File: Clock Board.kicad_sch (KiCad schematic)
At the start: 20 parts, among them SW1 Micro Push SPST, SW2 SW_SPDT, U1 NE555P, U2 NE555P, U3 NE555P, U4 74HCT02, U5 74HCT02, U6 74LS08

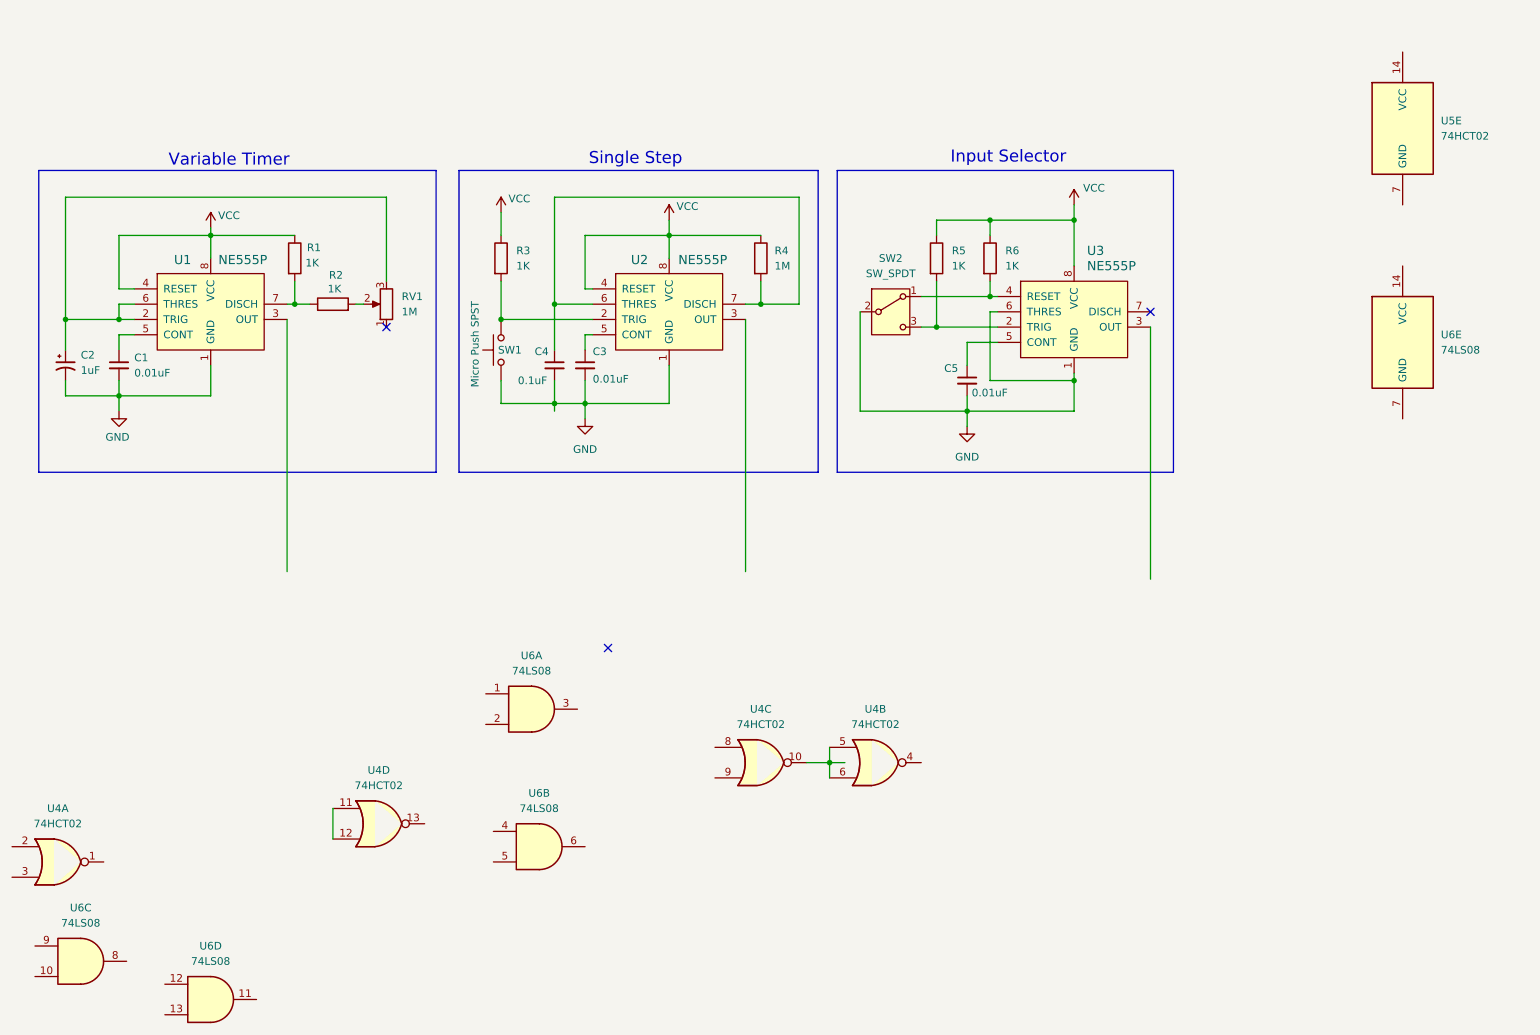
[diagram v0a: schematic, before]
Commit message: PCB Work
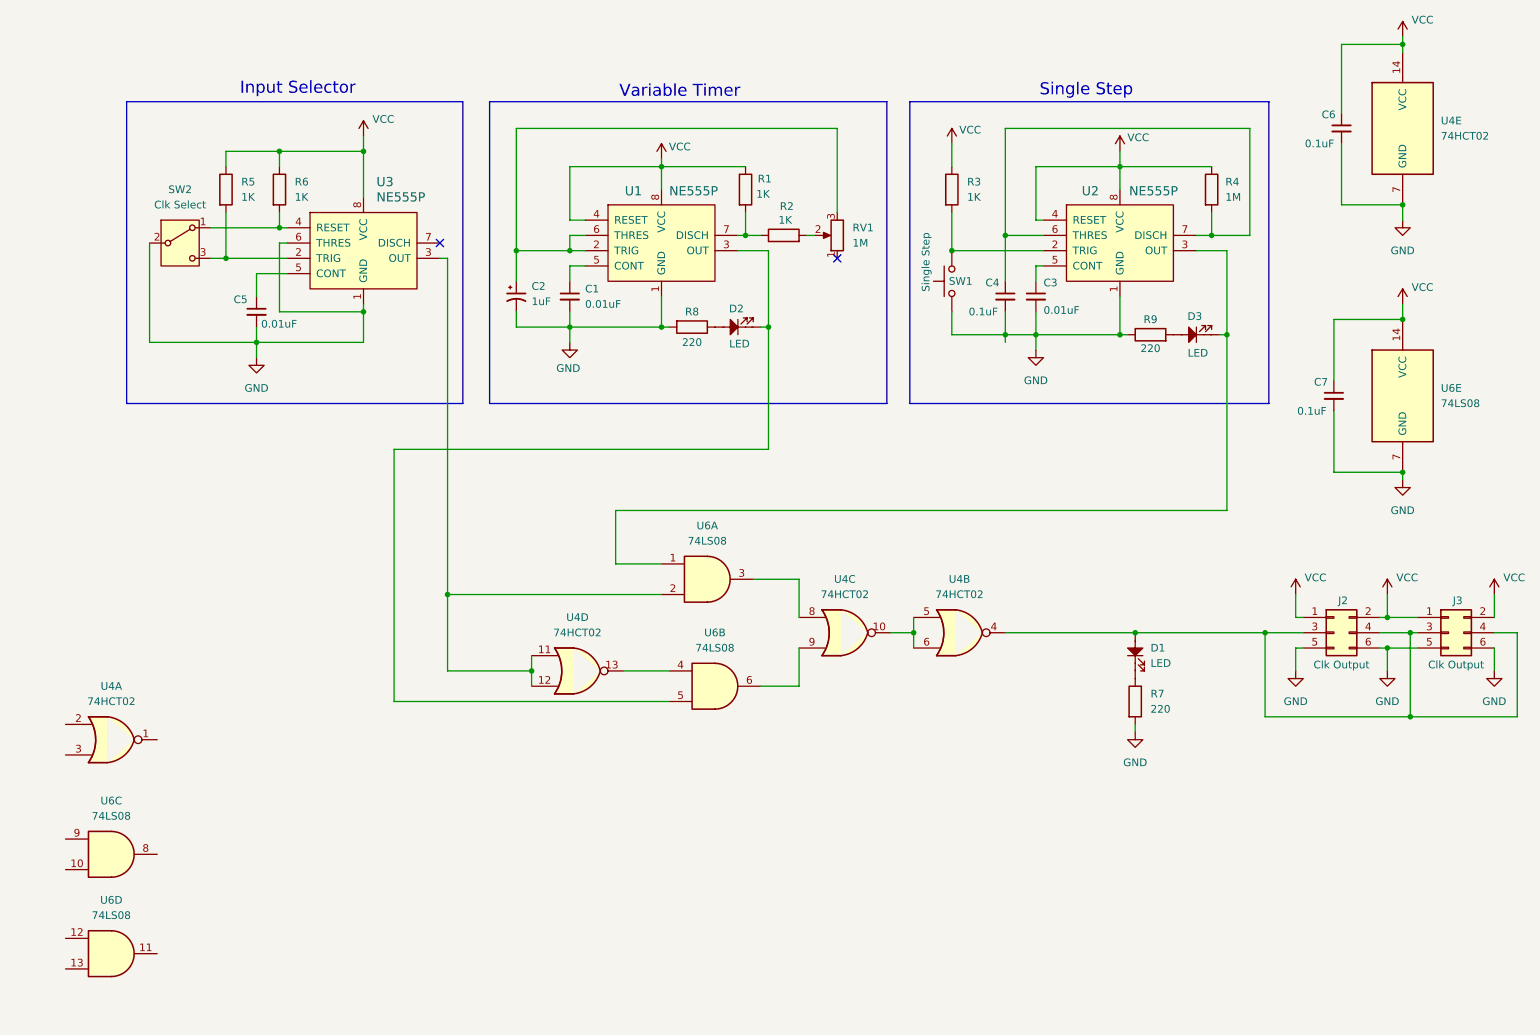
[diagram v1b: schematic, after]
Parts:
- added C6, C7: 0.1uF, Capacitor_THT:C_Disc_D5.0mm_W2.5mm_P5.00mm, symbol Device:C_Small
- added D1, D2, D3: LED, LED_THT:LED_D5.0mm, symbol PCM_SL_Devices:LED
- added J2: Clk Output, Connector_PinSocket_2.54mm:PinSocket_2x03_P2.54mm_Vertical, symbol Connector_Generic:Conn_02x03_Odd_Even
- added J3: Clk Output, Connector_PinHeader_2.54mm:PinHeader_2x03_P2.54mm_Vertical, symbol Connector_Generic:Conn_02x03_Odd_Even
- added R7, R8, R9: 220, Resistor_THT:R_Axial_DIN0207_L6.3mm_D2.5mm_P10.16mm_Horizontal, symbol Device:R
- C1, C3, C4, C5: footprint (none) -> Capacitor_THT:C_Disc_D5.0mm_W2.5mm_P5.00mm
- C2: footprint (none) -> PCM_Capacitor_THT_AKL:CP_Radial_D5.0mm_P2.00mm
- R1, R2, R3, R4, R5, R6: footprint (none) -> Resistor_THT:R_Axial_DIN0207_L6.3mm_D2.5mm_P10.16mm_Horizontal
- RV1: footprint (none) -> Potentiometer_THT:Potentiometer_TT_P0915N
- SW1: value Micro Push SPST -> Single Step; footprint (none) -> digikey-footprints:Terminal_Block_D1.3mm_P5mm
- SW2: value SW_SPDT -> Clk Select; footprint (none) -> Button_Switch_THT:SW_Slide_SPDT_Straight_CK_OS102011MS2Q
- U1, U2, U3: footprint digikey-footprints:DIP-8_W7.62mm -> Package_DIP:DIP-8_W7.62mm_Socket
- U4, U6: footprint (none) -> Package_DIP:DIP-14_W7.62mm_Socket
- U4: renamed from U5; footprint (none) -> Package_DIP:DIP-14_W7.62mm_Socket
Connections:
- net GND: now also U4.7 (GND), U6.7 (GND), C6.2, C7.2, J2.5 (Pin_5), J2.6 (Pin_6), J3.5 (Pin_5), J3.6 (Pin_6), R7.2, R8.2, R9.1
- net VCC: now also U4.14 (VCC), U6.14 (VCC), C6.1, C7.1, J2.1 (Pin_1), J2.2 (Pin_2), J3.1 (Pin_1), J3.2 (Pin_2)
- net at U1.3 (OUT): now also U6.5, D2.1
- net at U2.3 (OUT): now also U6.1, D3.1
- net at U6.2: now also U3.3 (OUT), U4.11, U4.12
- net at U6.3: now also U4.8
- net at U6.4: now also U4.13
- net at U6.6: now also U4.9
- net at U4.4: now also D1.2, J2.3 (Pin_3), J2.4 (Pin_4), J3.3 (Pin_3), J3.4 (Pin_4)
- new net: D3.2, R9.2
- new net: D2.2, R8.1
- new net: D1.1, R7.1
- no-connect marks 3 -> 2
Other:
- moved on the sheet: C1, C2, C3, C4, C5, R1, R2, R3, R4, R5, R6, RV1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
